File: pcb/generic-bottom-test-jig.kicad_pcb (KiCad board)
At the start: 2 copper layers, 36 x 36 mm, 13 parts

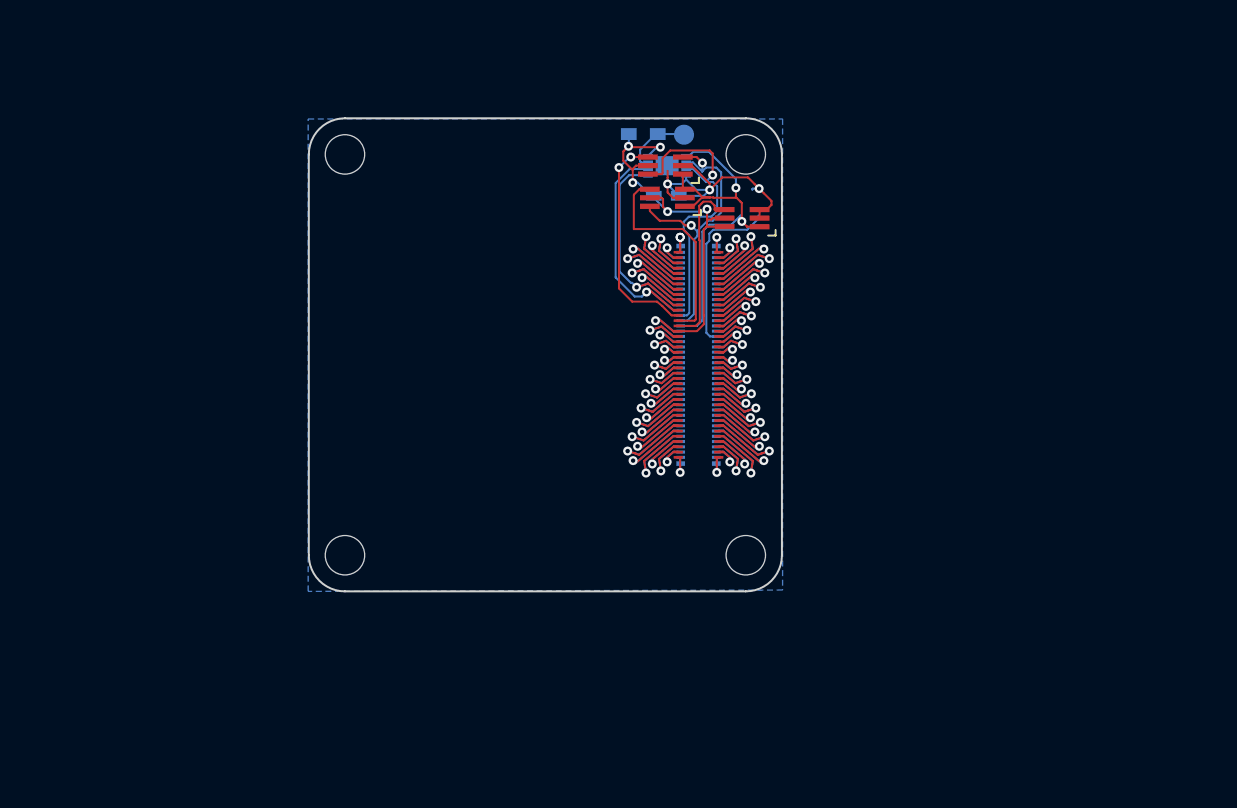
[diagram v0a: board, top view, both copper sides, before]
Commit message: Gerbers for v1 of the test jig.
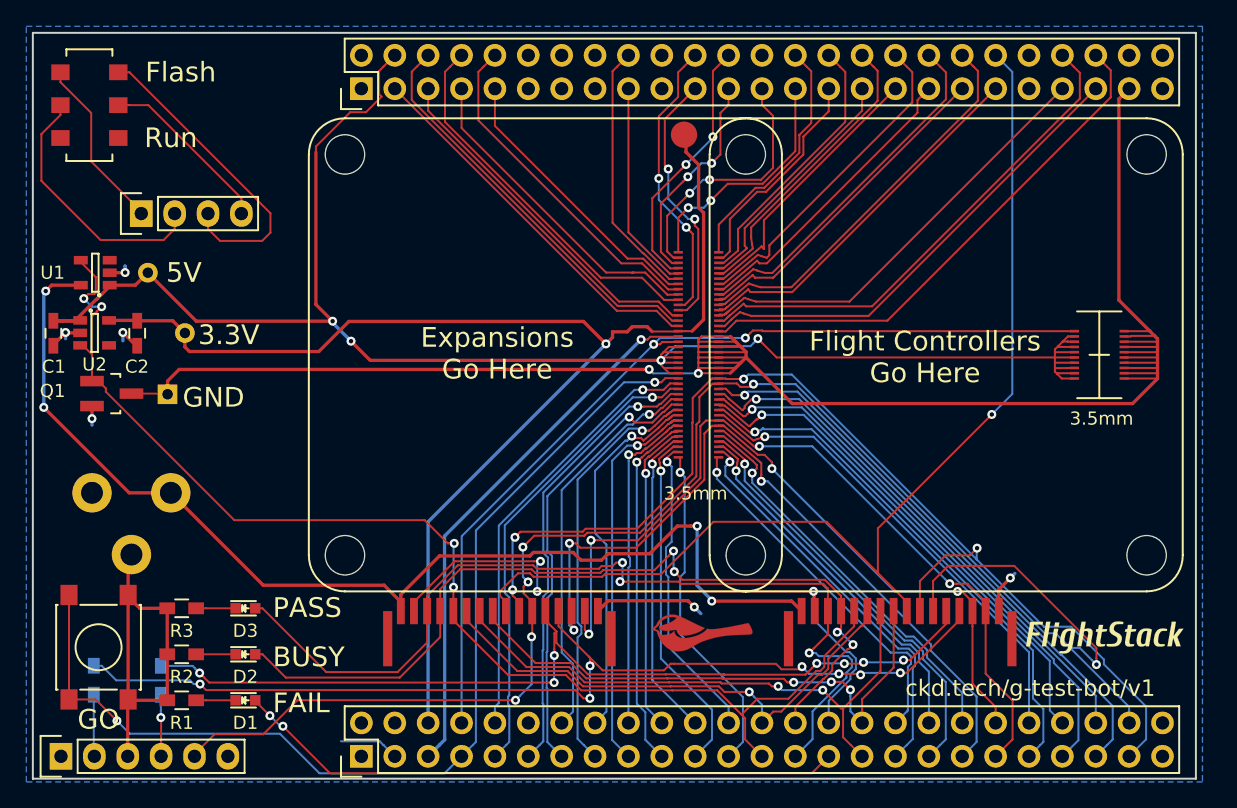
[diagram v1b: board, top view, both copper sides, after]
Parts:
- removed PORT_ANDOR1: SN74LVC1G0832, Housings_SOT-23_SOT-143_TSOT-6:SC-70-6_Handsoldering
- removed PORT_C1: 0.1uF, Capacitors_SMD:C_0603_HandSoldering
- removed PORT_IC1: AT24CS02-MAHM, Housings_DFN_QFN:DFN-8-1EP_3x2mm_Pitch0.5mm
- removed PORT_IN1: DF40-80pin-Header, DF40-80pin-Header
- removed PORT_INV1, PORT_XOR1: SN74LVC1G58, Housings_SOT-23_SOT-143_TSOT-6:SC-70-6_Handsoldering
- removed PORT_P1: CONN_01X01, Measurement_Points:Measurement_Point_Round-SMD-Pad_Small
- removed PORT_R1: 10k, Resistors_SMD:R_0603_HandSoldering
- added C1: 2.2uF, Capacitors_SMD:C_0603_HandSoldering, F.Cu at (110.6, 106.4)
- added C2: 1uF, Capacitors_SMD:C_0603_HandSoldering, F.Cu at (116.9, 106.4)
- added CON1: BARREL_JACK, barrel-jack:PJ-037BH-SMT, F.Cu at (116.5, 118.5)
- added D1: RED, LEDs:LED_0603, F.Cu at (125.2, 134.3)
- added D2: YELLOW, LEDs:LED_0603, F.Cu at (125.2, 130.8)
- added D3: GREEN, LEDs:LED_0603, F.Cu at (125.2, 127.3)
- added G***: Chickadee 3mm, chickadee:chickadee_3mm_fcu, F.Cu at (159.9, 129.2)
- added G***: LOGO, flightstack:flightstack-12mm, F.Cu at (190.6, 129.5)
- added P1: CONN_01X06, Pin_Headers:Pin_Header_Straight_1x06, F.Cu at (111.1, 138.6)
- added P10: CONN_01X01, Measurement_Points:Measurement_Point_Round-TH_Small, F.Cu at (120.6, 106.3)
- added P11: CONN_01X01, Measurement_Points:Measurement_Point_Square-TH_Small, F.Cu at (119.2, 111.0)
- added P2: CONN_02X25, Pin_Headers:Pin_Header_Straight_2x25, F.Cu at (134.0, 138.6)
- added P3: CONN_01X04, Pin_Headers:Pin_Header_Straight_1x04, F.Cu at (117.2, 97.2)
- added P4: CONN_02X25, Pin_Headers:Pin_Header_Straight_2x25, F.Cu at (134.0, 87.8)
- added P5: CONN_01X16, fci:SFW12LF-16pin, F.Cu at (144.5, 130.0)
- added P6: CONN_02X10, hirose-df40:DF40-1.5mm-20pin-Receptacle, F.Cu at (190.2, 108.0)
- added P7: CONN_01X01, mill-max-pogo-pin:0910, F.Cu at (158.6, 91.2)
- added P8: CONN_01X16, fci:SFW12LF-16pin, F.Cu at (175.0, 130.0)
- added P9: CONN_01X01, Measurement_Points:Measurement_Point_Round-TH_Small, F.Cu at (117.8, 101.8)
- added Q1: Q_NMOS_GSD, TO_SOT_Packages_SMD:SOT-23_Handsoldering, F.Cu at (115.0, 111.0)
- added R1: 1k, Resistors_SMD:R_0603_HandSoldering, F.Cu at (120.3, 134.3)
- added R2: 1k, Resistors_SMD:R_0603_HandSoldering, F.Cu at (120.3, 130.8)
- added R3: 1k, Resistors_SMD:R_0603_HandSoldering, F.Cu at (120.3, 127.3)
- added R4: 0, Resistors_SMD:R_0603_HandSoldering, B.Cu at (118.7, 132.8)
- added R5: 0, Resistors_SMD:R_0603_HandSoldering, B.Cu at (113.6, 132.8)
- added REF**: MountingHole_3mm, Mounting_Holes:MountingHole_3mm, F.Cu at (193.8, 123.2)
- added REF**: MountingHole_3mm, Mounting_Holes:MountingHole_3mm, F.Cu at (193.8, 92.8)
- added SW1: Switch_SPDT_x2, copal-electronics:CL-SB-22B, F.Cu at (113.3, 89.0)
- added SW2: SPST, Buttons_Switches_SMD:SW_SPST_PTS645, F.Cu at (114.0, 130.2)
- added U1: STMPS2151, TO_SOT_Packages_SMD:SOT-23-5, F.Cu at (113.8, 101.8)
- added U2: TLV70233DBV, TO_SOT_Packages_SMD:SOT-23-5, F.Cu at (113.7, 106.3)
- PORT_OUT1: value DF40-3-4mm-80pin-Receptacle -> CKD_SANDWICH; footprint DF40-3-4mm-80pin-Receptacle -> hirose-df40:DF40-3-4mm-80pin-Receptacle
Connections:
- PORT_OUT1 pad 1: (no net) -> /PD5
- PORT_OUT1 pad 10: (no net) -> /PC15
- PORT_OUT1 pad 11: (no net) -> /PB7_SDA
- PORT_OUT1 pad 12: (no net) -> /PB6_SCL
- PORT_OUT1 pad 13: (no net) -> /PF0
- PORT_OUT1 pad 14: (no net) -> /PF1
- PORT_OUT1 pad 15: (no net) -> /PF9
- PORT_OUT1 pad 16: (no net) -> /PC0_3V3
- PORT_OUT1 pad 17: (no net) -> /PC1_3V3_E
- PORT_OUT1 pad 18: (no net) -> /PC2_BATT
- PORT_OUT1 pad 19: (no net) -> /PF10_5V
- PORT_OUT1 pad 2: (no net) -> /PD7
- PORT_OUT1 pad 20: (no net) -> /PF10_5V
- PORT_OUT1 pad 21: (no net) -> /PF10_5V
- PORT_OUT1 pad 22: (no net) -> /PF10_5V
- PORT_OUT1 pad 23: (no net) -> /PF10_5V
- PORT_OUT1 pad 24: (no net) -> /PF10_5V
- PORT_OUT1 pad 25: (no net) -> /PC3_SWITCH
- PORT_OUT1 pad 26: (no net) -> /PF2
- PORT_OUT1 pad 27: (no net) -> /PA1
- PORT_OUT1 pad 28: (no net) -> /PA3
- PORT_OUT1 pad 29: (no net) -> /PA2
- PORT_OUT1 pad 3: (no net) -> /PB4
- PORT_OUT1 pad 30: (no net) -> /PF4
- PORT_OUT1 pad 31: (no net) -> /PA5_SCL
- PORT_OUT1 pad 32: (no net) -> /PA4
- PORT_OUT1 pad 33: (no net) -> /PA7_SDA
- PORT_OUT1 pad 34: (no net) -> /PA6_SDO
- PORT_OUT1 pad 35: (no net) -> /PC5
- PORT_OUT1 pad 36: (no net) -> /PC4
- PORT_OUT1 pad 37: (no net) -> /PB0
- PORT_OUT1 pad 38: (no net) -> /PB1
- PORT_OUT1 pad 39: (no net) -> /PB2
- PORT_OUT1 pad 4: (no net) -> /PB5
- PORT_OUT1 pad 40: (no net) -> /PE7
- PORT_OUT1 pad 41: (no net) -> /PD6
- PORT_OUT1 pad 42: (no net) -> /PD3
- PORT_OUT1 pad 43: (no net) -> /PD4
- PORT_OUT1 pad 44: (no net) -> /PD1
- PORT_OUT1 pad 45: (no net) -> /PD2
- PORT_OUT1 pad 46: (no net) -> /PC12
- PORT_OUT1 pad 47: (no net) -> /PD0
- PORT_OUT1 pad 48: (no net) -> /PC10
- PORT_OUT1 pad 49: (no net) -> /PC11
- PORT_OUT1 pad 5: (no net) -> /PB8
- PORT_OUT1 pad 50: (no net) -> /PA14_SWCLK
- PORT_OUT1 pad 51: (no net) -> /PA15
- PORT_OUT1 pad 52: (no net) -> /PF6
- PORT_OUT1 pad 53: (no net) -> /PA10
- PORT_OUT1 pad 54: (no net) -> /PA9
- PORT_OUT1 pad 55: (no net) -> /PA8
- PORT_OUT1 pad 56: (no net) -> /PC9
- PORT_OUT1 pad 57: (no net) -> /PC8_GND
- PORT_OUT1 pad 58: (no net) -> /PC8_GND
- PORT_OUT1 pad 59: (no net) -> /PC8_GND
- PORT_OUT1 pad 6: (no net) -> /PB9
- PORT_OUT1 pad 60: (no net) -> /PC8_GND
- PORT_OUT1 pad 61: (no net) -> /PC8_GND
- PORT_OUT1 pad 62: (no net) -> /PC8_GND
- PORT_OUT1 pad 63: (no net) -> /PC8_GND
- PORT_OUT1 pad 64: (no net) -> /PC8_GND
- PORT_OUT1 pad 65: (no net) -> /PC6_BOOT0
- PORT_OUT1 pad 66: (no net) -> /PC7_RESET
- PORT_OUT1 pad 67: (no net) -> /PD15
- PORT_OUT1 pad 68: (no net) -> /PD14
- PORT_OUT1 pad 69: (no net) -> /PD13
- PORT_OUT1 pad 7: (no net) -> /PE6
- PORT_OUT1 pad 70: (no net) -> /PD12
- PORT_OUT1 pad 71: (no net) -> /PD11
- PORT_OUT1 pad 72: (no net) -> /PD10
- PORT_OUT1 pad 73: (no net) -> /PD9_RX
- PORT_OUT1 pad 74: (no net) -> /PD8_TX
- PORT_OUT1 pad 75: (no net) -> /PB15
- PORT_OUT1 pad 76: (no net) -> /PB14
- PORT_OUT1 pad 77: (no net) -> /PB13
- PORT_OUT1 pad 78: (no net) -> /PB12
- PORT_OUT1 pad 79: (no net) -> /PB11
- PORT_OUT1 pad 8: (no net) -> /PC13
- PORT_OUT1 pad 80: (no net) -> /PB10
- PORT_OUT1 pad 9: (no net) -> /PC14
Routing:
- net (no net): track 470.7 -> 0.07 mm, vias 78 -> 0
- net /PC8_GND: track 0.00 -> 157.4 mm, vias 0 -> 2
- net /PF10_5V: track 0.00 -> 131.7 mm, vias 0 -> 4
- net /PC7_RESET: track 0.00 -> 126.9 mm, vias 0 -> 6
- net /PC0_3V3: track 0.00 -> 98.9 mm, vias 0 -> 1
- net /PE9_LD3_RED: track 0.00 -> 93.2 mm, vias 0 -> 4
- net /PC6_BOOT0: track 0.00 -> 86.0 mm, vias 0 -> 4
- net +5V: track 0.00 -> 85.5 mm, vias 0 -> 4
- net /PA13_SWDIO: track 0.00 -> 82.4 mm, vias 0 -> 1
- net /PC3_SWITCH: track 0.00 -> 78.5 mm, vias 0 -> 2
- net /SWCLK: track 0.00 -> 78.2 mm, vias 0 -> 7
- net /PE11_LD7_GREEN: track 0.00 -> 71.3 mm, vias 0 -> 3
- net /SWDIO: track 0.00 -> 70.4 mm, vias 0 -> 7
- net /PC2_BATT: track 0.00 -> 69.3 mm, vias 0 -> 2
- net /PE10_LD5_ORANGE: track 0.00 -> 66.4 mm, vias 0 -> 4
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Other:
- board size 36 x 36 mm -> 88.5 x 56.8 mm
- net class Default: clearance 0.1524 -> 0.14986
- net class Power added: clearance 0.14986, trace_width 0.254, via_dia 0.6858, via_drill 0.3302
- rule trace_clearance: 0.1524 -> 0.14986
- board text added: "3.3V"
- board text added: "3.5mm"
- board text added: "5V"
- board text added: "BUSY"
- board text added: "Expansions Go Here"
- board text added: "FAIL"
- board text added: "Flash"
- board text added: "Flight Controllers Go Here"
- board text added: "GND"
- board text added: "GO"
- board text added: "PASS"
- board text added: "Run"
- board text added: "This side intentionally left blank. (Its the back.)"
- board text added: "ckd.tech/g-test-bot/v1"
